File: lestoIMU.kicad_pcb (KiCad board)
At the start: 2 copper layers, 20 x 20 mm, 16 parts, among them J1 PRG, J2 PWR, J3 RST, J4 PRG, U1 ESP-12E, U2 BMI160

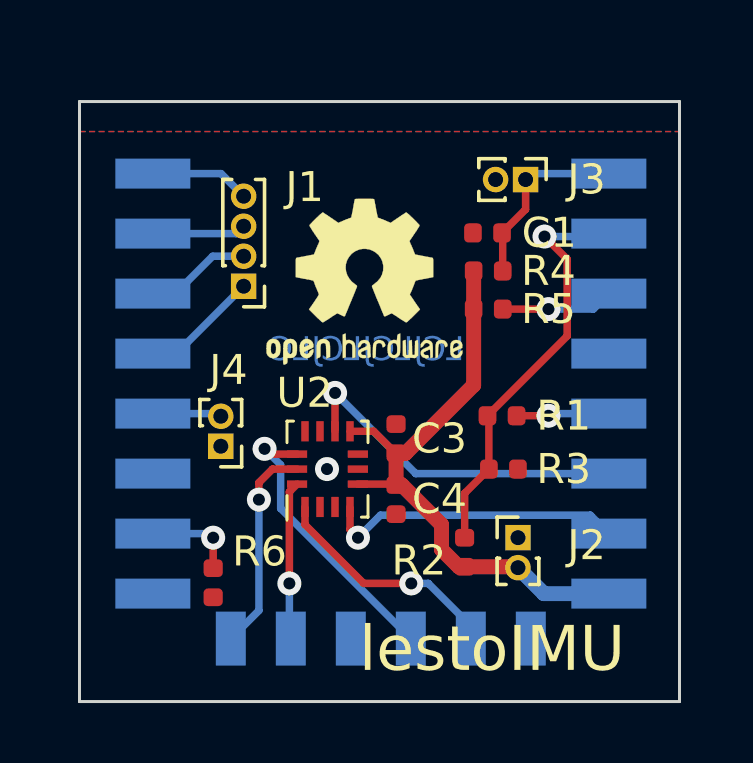
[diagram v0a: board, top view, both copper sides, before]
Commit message: major update
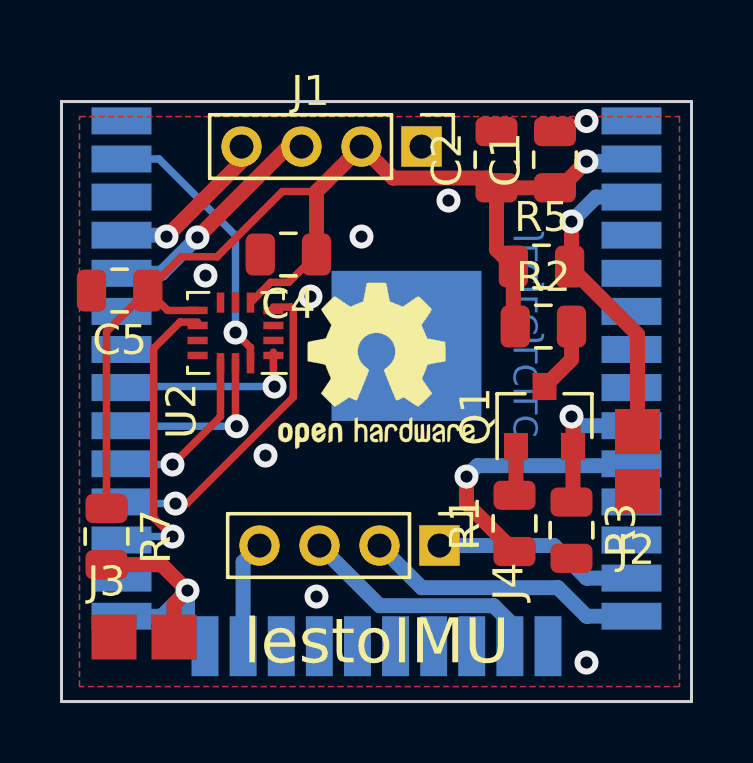
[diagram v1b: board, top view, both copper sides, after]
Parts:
- removed C3: 100nf, Capacitor_SMD:C_0402_1005Metric
- removed the J3 at (134.9, 62.6)
- removed R4: 10K, Resistor_SMD:R_0402_1005Metric
- removed R6: 1K, Resistor_SMD:R_0402_1005Metric
- added C2: 100nF, Capacitor_SMD:C_0805_2012Metric, F.Cu at (133.9, 61.9)
- added C4: 100nf, Capacitor_SMD:C_0805_2012Metric, F.Cu at (127.0, 65.1)
- added J4: JTAG, Connector_PinHeader_2.00mm:PinHeader_1x04_P2.00mm_Vertical, F.Cu at (132.0, 74.8)
- added Q1: Q_NMOS_GSD, Package_TO_SOT_SMD:SOT-23, F.Cu at (135.5, 70.5)
- added R7: 10K, Resistor_SMD:R_0805_2012Metric, F.Cu at (120.9, 74.5)
- C1: value 100nF -> 22uF; footprint Capacitor_SMD:C_0402_1005Metric -> Capacitor_SMD:C_0805_2012Metric
- C5: renamed from C4; footprint Capacitor_SMD:C_0402_1005Metric -> Capacitor_SMD:C_0805_2012Metric
- J1: footprint Connector_PinHeader_1.00mm:PinHeader_1x04_P1.00mm_Vertical -> Connector_PinHeader_2.00mm:PinHeader_1x04_P2.00mm_Vertical
- J2: value PWR -> RST; footprint Connector_PinHeader_1.00mm:PinHeader_1x02_P1.00mm_Vertical -> lestoConnector:PinHeader_smd_bridge_1x02_P2.00mm_SMD
- J3: renamed from J4; footprint Connector_PinHeader_1.00mm:PinHeader_1x02_P1.00mm_Vertical -> lestoConnector:PinHeader_smd_bridge_1x02_P2.00mm_SMD
- R1, R2, R3: footprint Resistor_SMD:R_0402_1005Metric -> Resistor_SMD:R_0805_2012Metric
- R5: value 1K -> 10K; footprint Resistor_SMD:R_0402_1005Metric -> Resistor_SMD:R_0805_2012Metric
- U1: value ESP-12E -> ESP32-WROOM-32D; footprint RF_Module:ESP-12E -> RF_Module:ESP32-WROOM-32
- moved C5 11.6 mm to (121.3, 66.3), turned to 180 degrees
- moved R2 7.97 mm to (135.5, 67.5), turned to 0 degrees
- moved J1 7.54 mm to (131.4, 61.5), turned to 270 degrees
- moved J3 6.83 mm to (122.1, 77.8), turned to 90 degrees
- moved U2 5.48 mm to (125.2, 67.7), turned to 180 degrees
- moved J2 4.65 mm to (138.6, 72.0), turned to 180 degrees
- moved R1 3.61 mm to (134.5, 74.1), turned to 90 degrees
- moved C1 3.32 mm to (135.8, 61.9), turned to 90 degrees
- moved R3 3.05 mm to (136.4, 74.3), turned to 270 degrees
- moved U1 3.00 mm to (129.9, 68.9)
- moved LOGO1 2.83 mm to (129.9, 68.8)
- moved R5 2.27 mm to (135.4, 65.5)
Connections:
- C1 pad 1: RESET -> +3V3
- J1 pad 1: Net-(J1-Pad1) -> GND
- J1 pad 2: Net-(J1-Pad2) -> +3V3
- J1 pad 3: Net-(J1-Pad3) -> RX
- J1 pad 4: Net-(J1-Pad4) -> TX
- J2 pad 2: +3V3 -> ENABLE
- J3 pad 2: GPIO0 -> BOOT
- R1 pad 1: GPIO14 -> EN_ADC
- R1 pad 2: ADC -> Net-(Q1-Pad1)
- R2 pad 2: ADC -> Net-(Q1-Pad3)
- U1 pad 1: RESET -> GND
- U1 pad 10: MISO -> EN_ADC
- U1 pad 11: CS -> Net-(U1-Pad11)
- U1 pad 13: MOSI -> MTMS
- U1 pad 14: CLK -> MTDI
- U1 pad 16: GPIO15 -> MTCK
- U1 pad 18: GPIO0 -> Net-(U1-Pad18)
- U1 pad 19: Net-(J1-Pad1) -> Net-(U1-Pad19)
- U1 pad 2: ADC -> +3V3
- U1 pad 20: Net-(J1-Pad2) -> Net-(U1-Pad20)
- U1 pad 21: Net-(J1-Pad3) -> Net-(U1-Pad21)
- U1 pad 22: Net-(J1-Pad4) -> Net-(U1-Pad22)
- U1 pad 5: GPIO14 -> Net-(U1-Pad5)
- U1 pad 6: INT2 -> Net-(U1-Pad6)
- U1 pad 7: INT1 -> Net-(U1-Pad7)
- U1 pad 8: +3V3 -> Net-(U1-Pad8)
- U1 pad 9: Net-(U1-Pad9) -> ADC
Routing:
- net +3V3: track 20.6 -> 38.7 mm, vias 0 -> 1
- net BOOT: track 0.00 -> 9.45 mm, vias 0 -> 1
- net MTDI: track 0.00 -> 9.38 mm
- net ADC: track 14.0 -> 5.02 mm
- net EN_ADC: track 0.00 -> 8.84 mm, vias 0 -> 1
- net MTCK: track 0.00 -> 8.21 mm
- net RX: track 0.00 -> 7.75 mm, vias 0 -> 1
- net MTMS: track 0.00 -> 6.85 mm
- net ENABLE: track 3.75 -> 10.3 mm
- net RESET: track 6.24 -> 0.00 mm
- net TX: track 0.00 -> 5.55 mm, vias 0 -> 1
- net MOSI: track 5.28 -> 9.32 mm
- net Net-(J1-Pad1): track 3.96 -> 0.00 mm
- net CS: track 9.50 -> 5.85 mm
- net MTDO: track 0.00 -> 3.58 mm
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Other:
- board size 20 x 20 mm -> 21 x 20 mm
